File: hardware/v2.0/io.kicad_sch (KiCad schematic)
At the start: 1 part, among them U1 ECP5U-25F-CABGA256

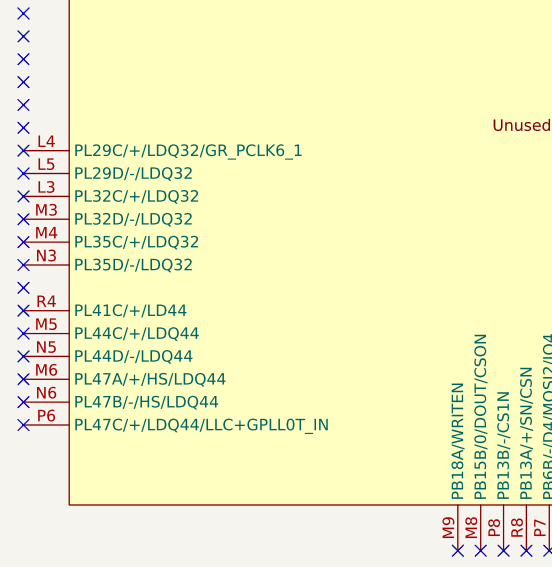
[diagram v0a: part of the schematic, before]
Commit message: ADC lines
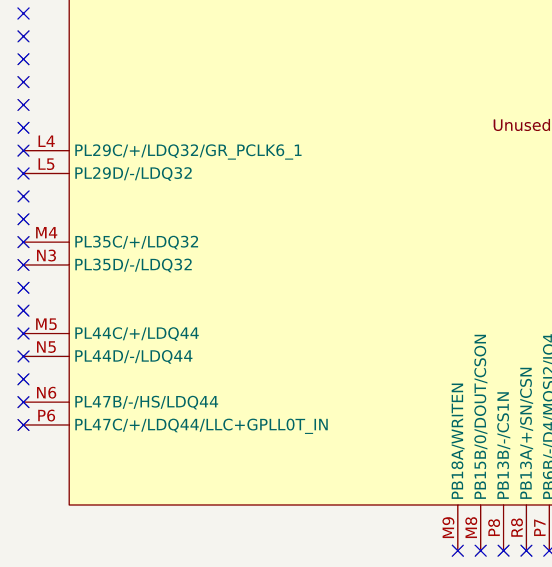
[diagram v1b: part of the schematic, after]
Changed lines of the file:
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@@
-					(unit 10)
-				)
-				(path "/f88da08e-cf42-4d03-a08f-3f602fe6658d/b5a9aa02-311b-4a9a-a7d4-646f15cdd9c2"
-					(reference "U1")
 					(unit 10)
 				)

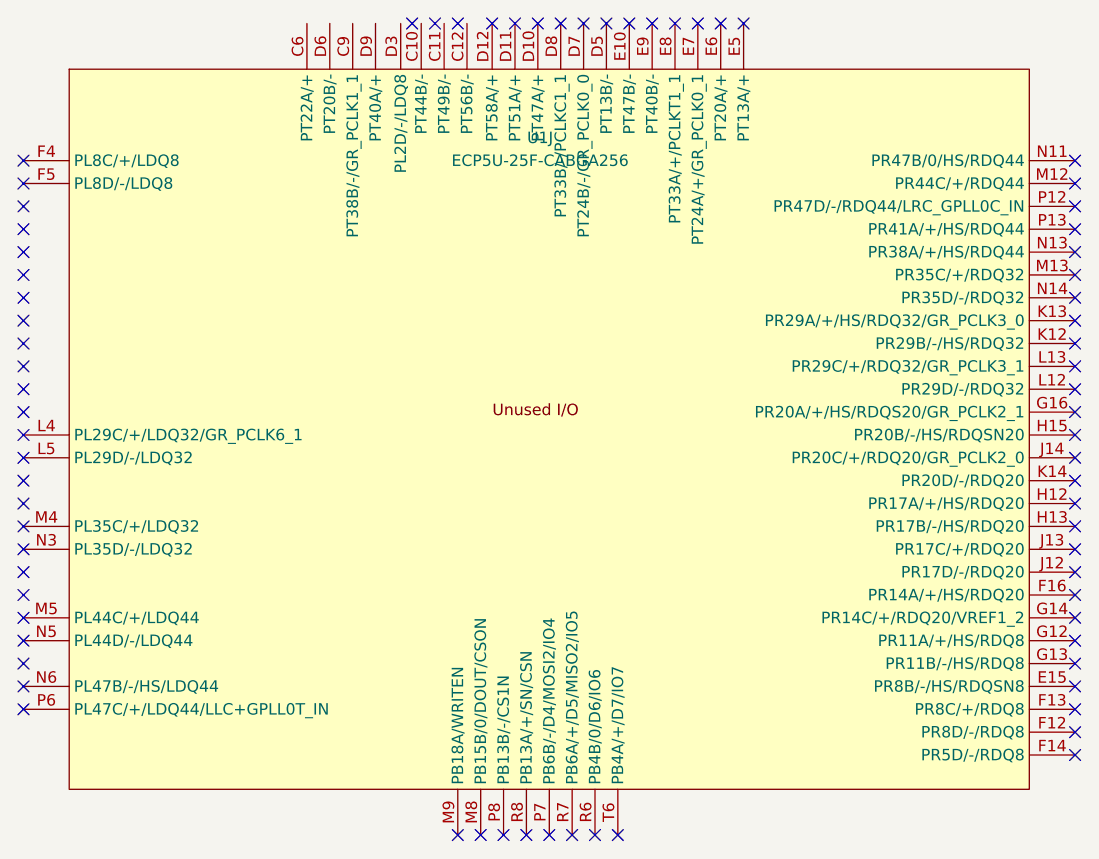
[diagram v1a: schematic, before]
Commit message: ADC CLKOUT±
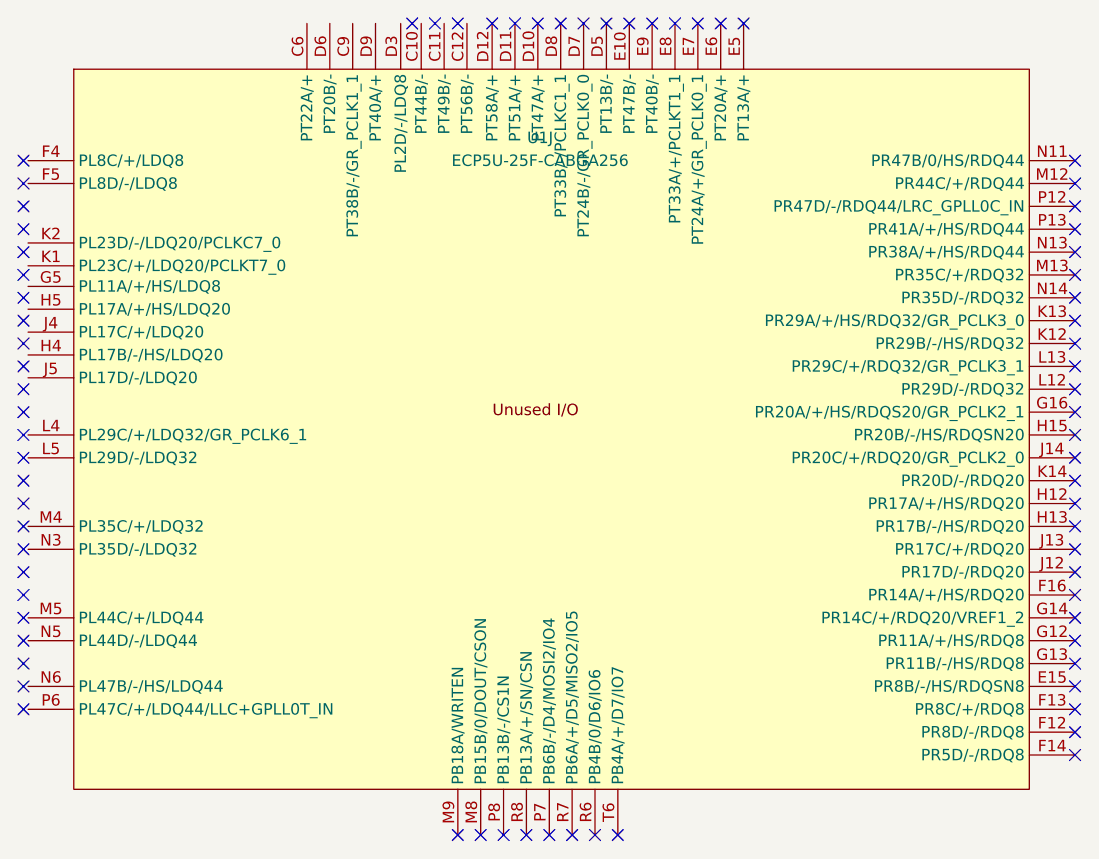
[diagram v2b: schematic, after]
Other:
- company: Chengyin Yao (cheyao), Vadym Vikulin -> Vadym Vikulin, Chengyin Yao (cheyao)
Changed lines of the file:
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@@
 	(title_block
 		(title "Icepi Zero")
-		(date "2026-01-05")
-		(rev "v2.0")
-		(company "Chengyin Yao (cheyao), Vadym Vikulin")
-		(comment 1 "https://github.com/cheyao/icepi-zero")
+		(date "2026-01-17")
+		(rev "v2.1")
+		(company "Vadym Vikulin, Chengyin Yao (cheyao)")
+		(comment 1 "https://github.com/vikulin/icepi-zero")
 		(comment 2 "License: Solderpad")
 		(comment 9 "OSHWA FR000026")
@@
 		(pin "P11"
 		)
+		(pin "N6"
+		)
 		(instances
